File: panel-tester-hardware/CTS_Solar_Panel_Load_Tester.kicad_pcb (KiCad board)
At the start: 2 copper layers, 60.1 x 70.5 mm, 12 parts, among them J1 Screw_Terminal_01x02, J2 Conn_01x02_Pin, J3 Conn_01x07, U1 INA219AxD, U2 YAAJ_BluePill

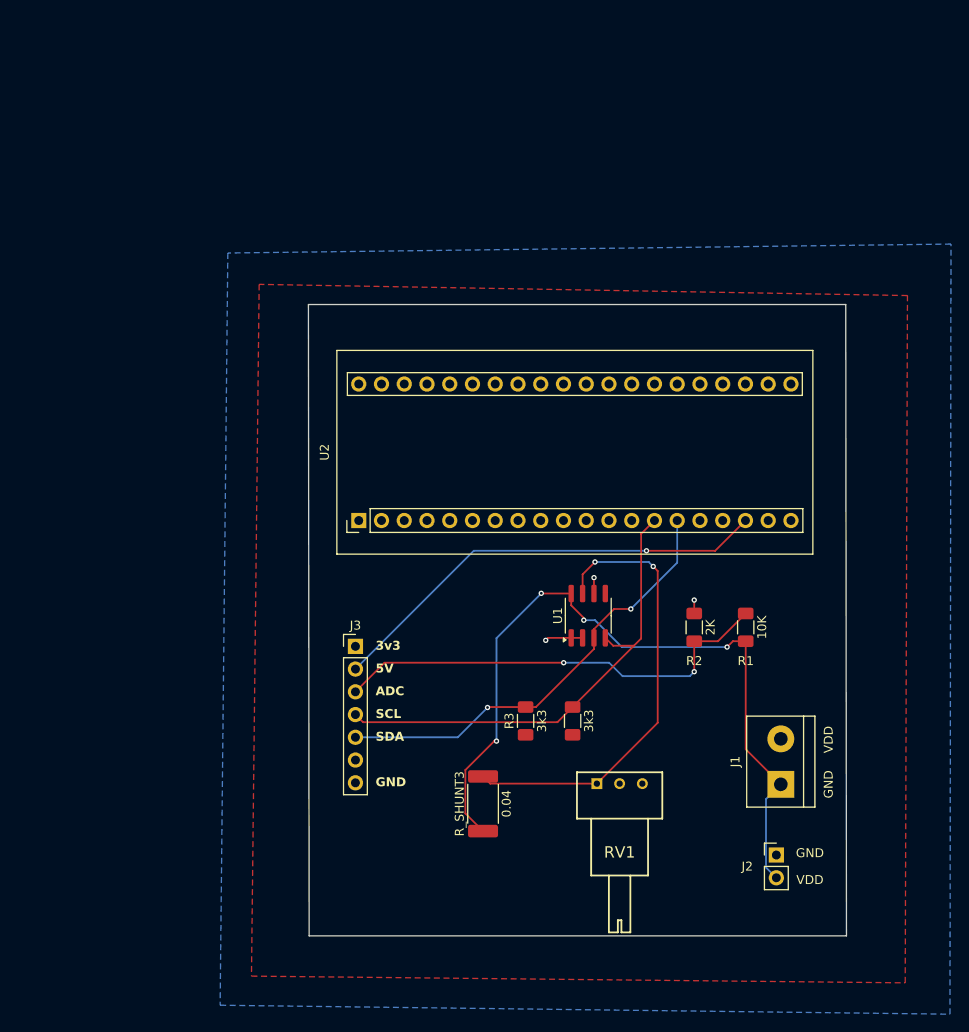
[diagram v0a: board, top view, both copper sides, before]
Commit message: Revert "Bluepill layout edits"
This reverts commit 7404dadbf005f9dc7929b7ea0254307db19fd9e4.
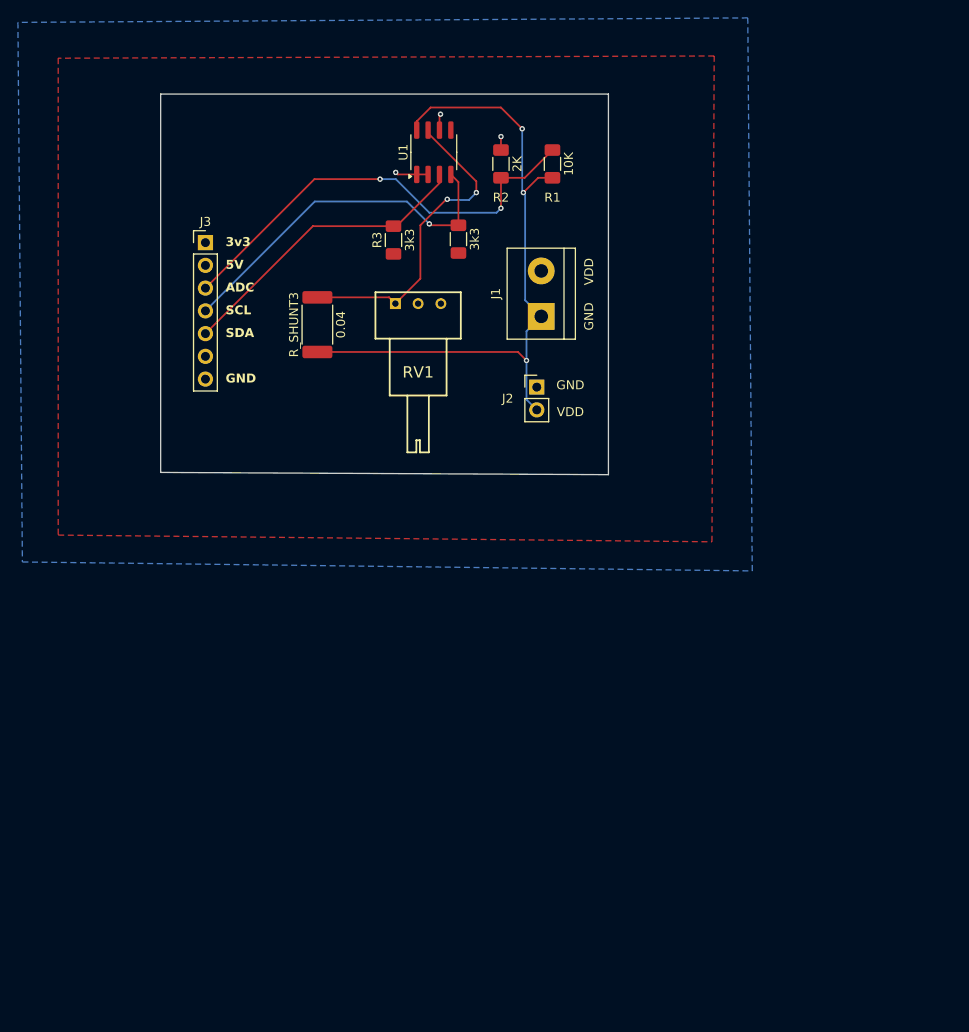
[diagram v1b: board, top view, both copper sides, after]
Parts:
- removed U2: YAAJ_BluePill, BluePill:YAAJ_BluePill_2
- moved J1 58.7 mm to (117.5, 57.3)
- moved J2 58.7 mm to (117.0, 65.2)
- moved RV1 58.1 mm to (101.2, 55.9)
- moved R_SHUNT3 56.6 mm to (92.5, 58.2)
- moved R1 56.1 mm to (118.8, 40.3)
- moved R2 56.1 mm to (113.0, 40.3)
- moved R3 55.7 mm to (101.0, 48.8)
- moved R4 55.3 mm to (108.2, 48.7)
- moved U1 54.5 mm to (105.5, 39.0)
- moved J3 48.1 mm to (80.0, 49.1)
- moved G*** 31.3 mm to (83.8, 36.2)
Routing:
- net +5V: track 50.9 -> 0.00 mm, vias 1 -> 0
- net MCU_I2C_SDA: track 50.0 -> 34.1 mm, vias 2 -> 0
- net Net-(U1-IN-): track 51.1 -> 35.9 mm
- net MCU_I2C_SCL: track 53.5 -> 40.4 mm, vias 0 -> 1
- net V_SOLAR_INPUT_POS: track 86.7 -> 75.6 mm, vias 4 -> 3
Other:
- board size 60.1 x 70.5 mm -> 50 x 42.5 mm
